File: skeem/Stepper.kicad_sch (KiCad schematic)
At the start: 7 parts, among them J3 JST XH 5 pin, M1 Stepper_hour, M1 Stepper_minute, U6 DRV8428, U7 DRV8428

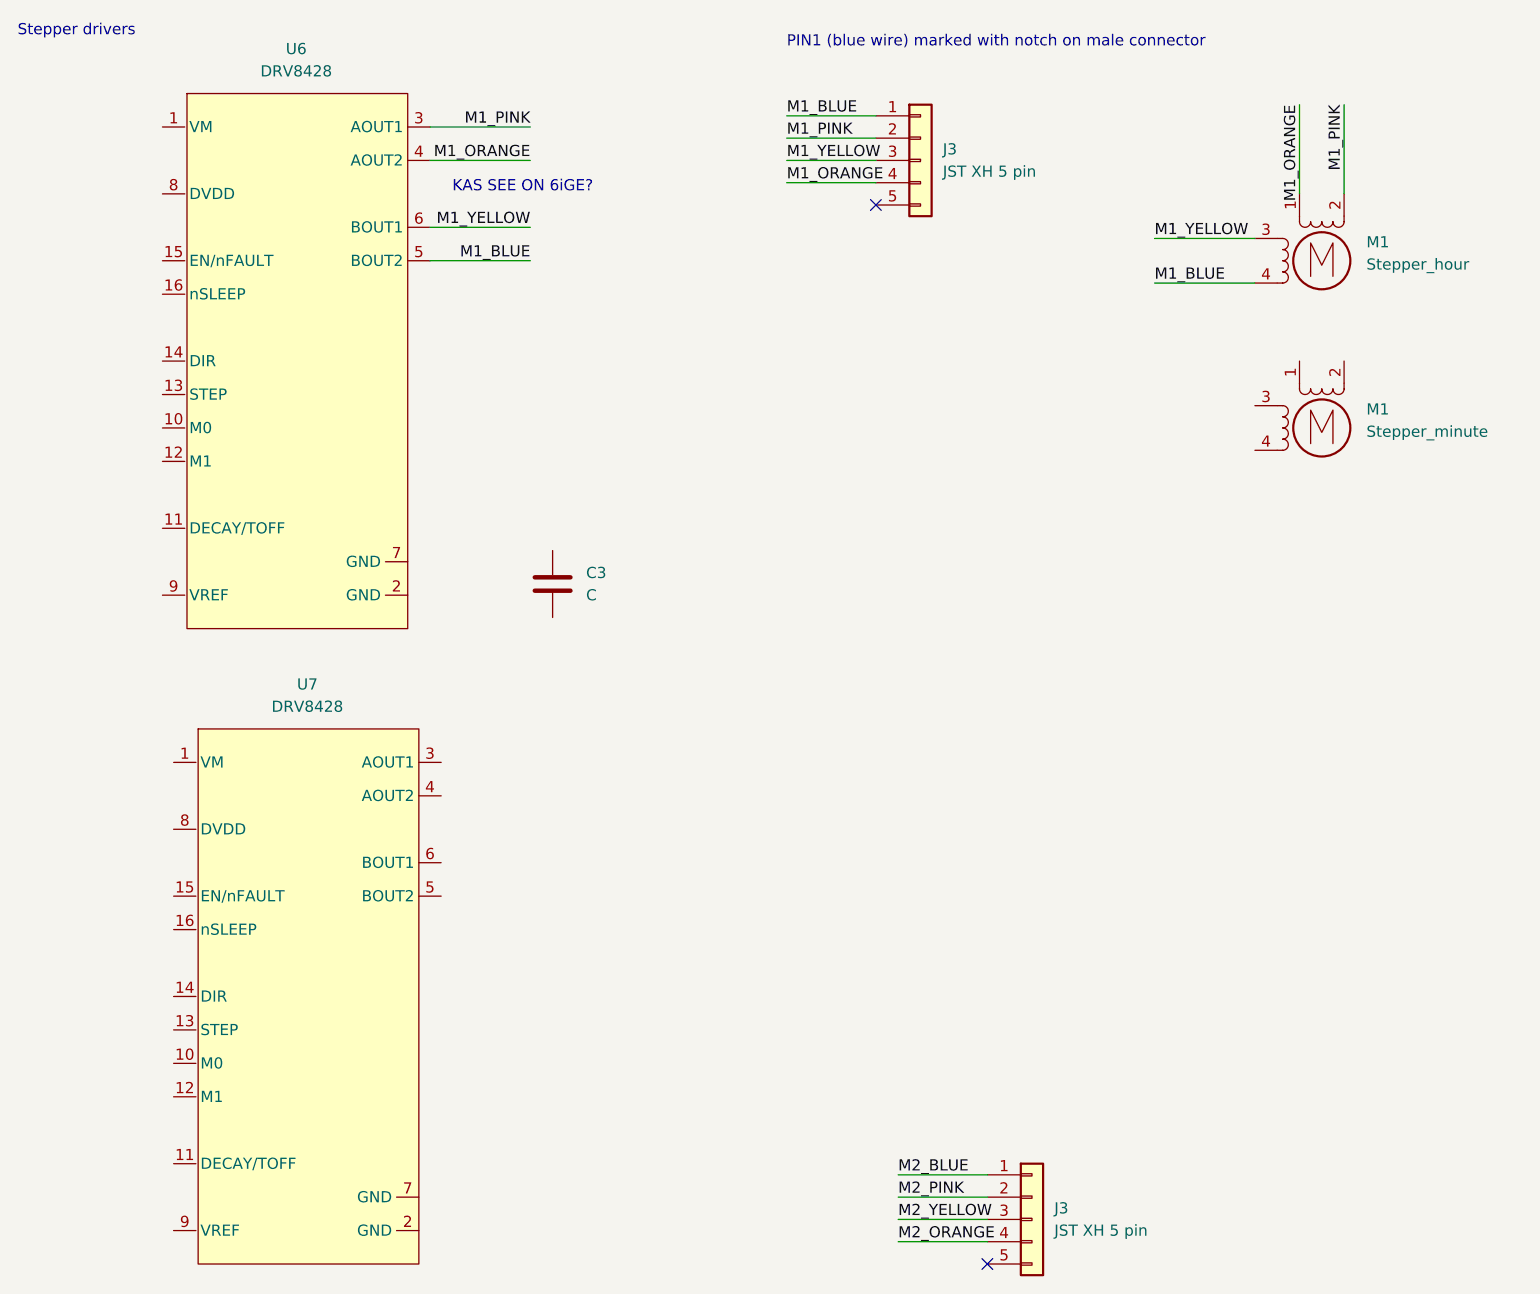
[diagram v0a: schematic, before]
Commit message: power mgmt
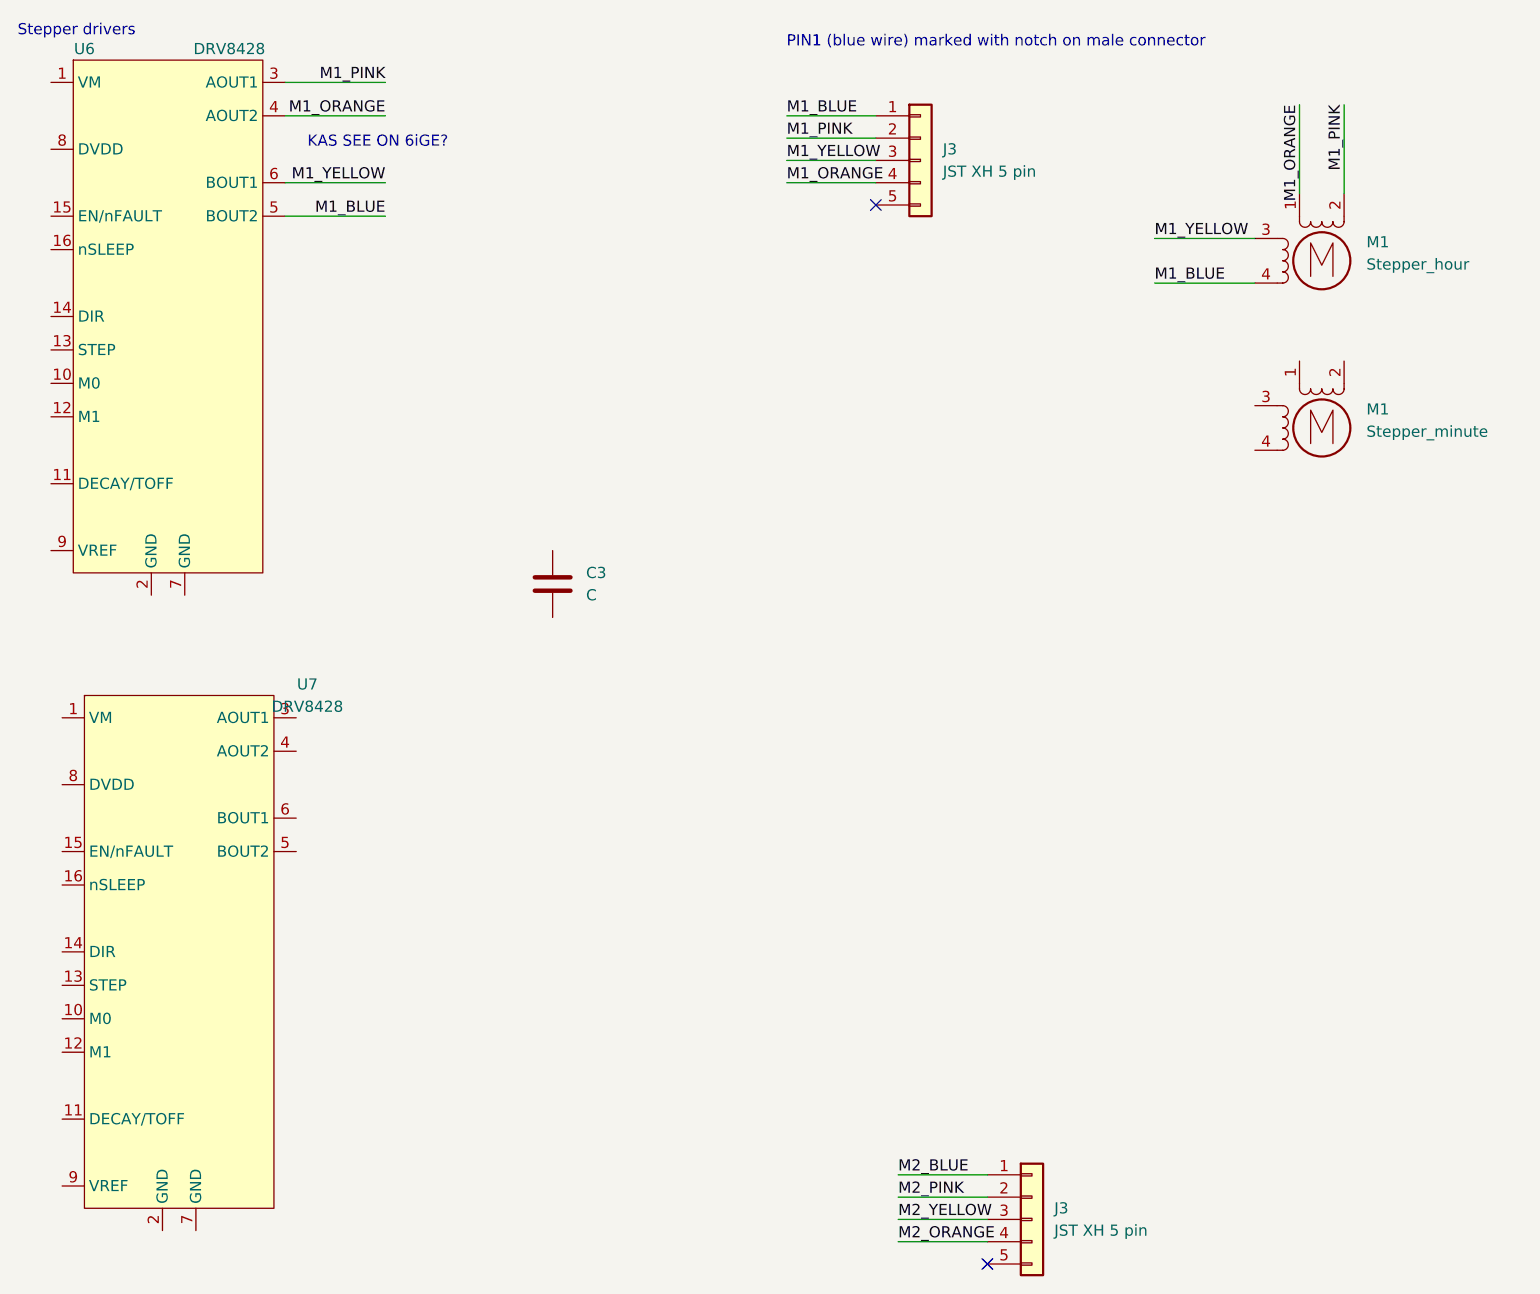
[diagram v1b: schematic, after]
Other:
- moved on the sheet: U6, U7
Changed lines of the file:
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@@
     (stroke (width 0) (type default))
   )
-  (wire (pts (xy 67.31 29.21) (xy 78.74 29.21))
+  (wire (pts (xy 50.8 24.13) (xy 62.23 24.13))
     (stroke (width 0) (type default))
   )
@@
     (stroke (width 0) (type default))
   )
-  (wire (pts (xy 67.31 33.02) (xy 78.74 33.02))
+  (wire (pts (xy 50.8 27.94) (xy 62.23 27.94))
     (stroke (width 0) (type default))
   )
@@
     (stroke (width 0) (type default))
   )
-  (wire (pts (xy 67.31 44.45) (xy 78.74 44.45))
+  (wire (pts (xy 50.8 39.37) (xy 62.23 39.37))
     (stroke (width 0) (type default))
   )
-  (wire (pts (xy 67.31 40.64) (xy 78.74 40.64))
+  (wire (pts (xy 50.8 35.56) (xy 62.23 35.56))
     (stroke (width 0) (type default))
   )
@@
     (effects (font (size 1.27 1.27)) (justify left bottom))
   )
-  (text "KAS SEE ON 6iGE?" (at 69.85 36.83 0)
+  (text "KAS SEE ON 6iGE?" (at 53.34 31.75 0)
     (effects (font (size 1.27 1.27)) (justify left bottom))
   )
@@
     (effects (font (size 1.27 1.27)) (justify left bottom))
   )
-  (label "M1_YELLOW" (at 78.74 40.64 180) (fields_autoplaced)
+  (label "M1_YELLOW" (at 62.23 35.56 180) (fields_autoplaced)
     (effects (font (size 1.27 1.27)) (justify right bottom))
   )
@@
     (effects (font (size 1.27 1.27)) (justify left bottom))
   )
-  (label "M1_PINK" (at 78.74 29.21 180) (fields_autoplaced)
+  (label "M1_PINK" (at 62.23 24.13 180) (fields_autoplaced)
     (effects (font (size 1.27 1.27)) (justify right bottom))
   )
@@
     (effects (font (size 1.27 1.27)) (justify left bottom))
   )
-  (label "M1_ORANGE" (at 78.74 33.02 180) (fields_autoplaced)
+  (label "M1_ORANGE" (at 62.23 27.94 180) (fields_autoplaced)
     (effects (font (size 1.27 1.27)) (justify right bottom))
   )
@@
     (effects (font (size 1.27 1.27)) (justify left bottom))
   )
-  (label "M1_BLUE" (at 78.74 44.45 180) (fields_autoplaced)
+  (label "M1_BLUE" (at 62.23 39.37 180) (fields_autoplaced)
     (effects (font (size 1.27 1.27)) (justify right bottom))
   )
@@
   )
   (symbol (lib_id "RVP_TopeltKell:DRV8428") (at 26.67 21.59 0) (unit 1)
-    (in_bom yes) (on_board yes) (dnp no) (fields_autoplaced)
-    (property "Reference" "U6" (at 52.07 20.32 0)
+    (in_bom yes) (on_board yes) (dnp no)
+    (property "Reference" "U6" (at 27.94 20.32 0)
       (effects (font (size 1.27 1.27)))
     )
-    (property "Value" "DRV8428" (at 52.07 22.86 0)
+    (property "Value" "DRV8428" (at 44.45 20.32 0)
       (effects (font (size 1.27 1.27)))
     )
